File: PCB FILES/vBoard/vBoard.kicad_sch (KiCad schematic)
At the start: 209 parts, among them SW1 SW_Push, SW10 SW_Push, SW11 SW_Push, SW12 SW_Push, SW13 SW_Push, SW14 SW_Push, SW15 SW_Push, SW16 SW_Push, SW17 SW_Push, SW18 SW_Push, SW19 SW_Push, SW2 SW_Push, SW20 SW_Push, SW21 SW_Push, SW22 SW_Push, SW23 SW_Push, SW24 SW_Push, SW25 SW_Push, SW26 SW_Push, SW27 SW_Push, SW28 SW_Push, SW29 SW_Push, SW3 SW_Push, SW30 SW_Push, SW31 SW_Push, SW32 SW_Push, SW33 SW_Push, SW34 SW_Push, SW35 SW_Push, SW36 SW_Push, SW37 SW_Push, SW38 SW_Push, SW39 SW_Push, SW4 SW_Push, SW40 SW_Push, SW41 SW_Push, SW42 SW_Push, SW43 SW_Push, SW44 SW_Push, SW45 SW_Push, SW46 SW_Push, SW47 SW_Push, SW48 SW_Push, SW49 SW_Push, SW5 SW_Push, SW50 SW_Push, SW51 SW_Push, SW52 SW_Push, SW53 SW_Push, SW54 SW_Push, SW55 SW_Push, SW56 SW_Push, SW57 SW_Push, SW58 SW_Push, SW59 SW_Push, SW6 SW_Push, SW60 SW_Push, SW61 SW_Push, SW62 SW_Push, SW63 SW_Push, SW64 SW_Push, SW65 SW_Push, SW66 SW_Push, SW67 SW_Push, SW68 SW_Push, SW69 SW_Push, SW7 SW_Push, SW70 SW_Push, SW71 SW_Push, SW72 SW_Push, SW73 SW_Push, SW74 SW_Push, SW75 SW_Push, SW76 SW_Push, SW77 SW_Push, SW78 SW_Push, SW79 SW_Push, SW8 SW_Push, SW80 SW_Push, SW81 SW_Push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

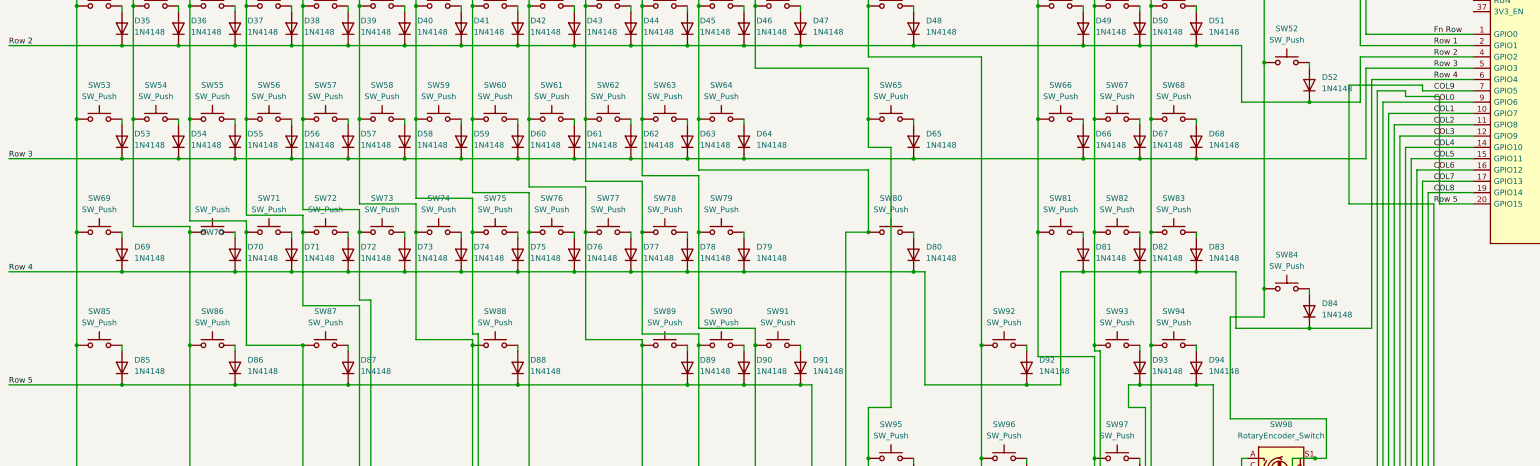
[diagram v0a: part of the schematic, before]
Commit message: DRC fixes.
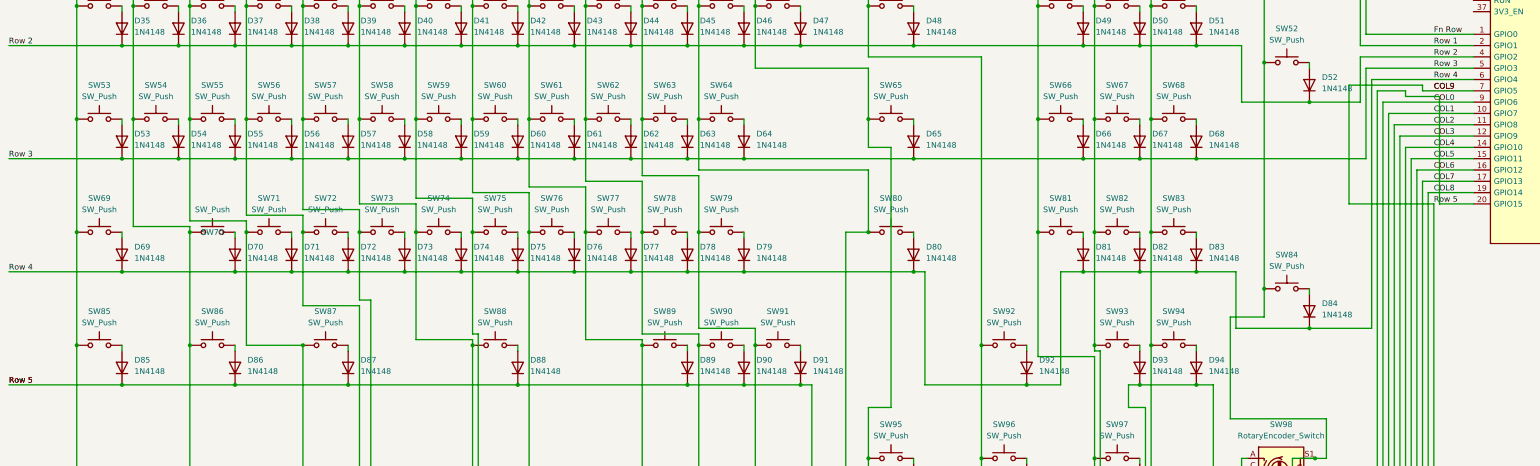
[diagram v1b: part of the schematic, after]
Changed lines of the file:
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@@
+		)
+	)
+	(label "COL9"
+		(at 332.74 99.06 0)
+		(effects
+			(font
+				(size 1.27 1.27)
+			)
+			(justify left bottom)
 		)
 	)
@@
 		)
 	)
+	(label "COL12"
+		(at 218.44 17.78 0)
+		(effects
+			(font
+				(size 1.27 1.27)
+			)
+			(justify left bottom)
+		)
+	)
+	(label "Row 5"
+		(at 12.7 165.1 0)
+		(effects
+			(font
+				(size 1.27 1.27)
+			)
+			(justify left bottom)
+		)
+	)
+	(label "COL14"
+		(at 243.84 17.78 0)
+		(effects
+			(font
+				(size 1.27 1.27)
+			)
+			(justify left bottom)
+		)
+	)
+	(label "Fn Row"
+		(at 332.74 86.36 0)
+		(effects
+			(font
+				(size 1.27 1.27)
+			)
+			(justify left bottom)
+		)
+	)
+	(label "COL5"
+		(at 332.74 114.3 0)
+		(effects
+			(font
+				(size 1.27 1.27)
+			)
+			(justify left bottom)
+		)
+	)
+	(label "COL11"
+		(at 392.43 91.44 0)
+		(effects
+			(font
+				(size 1.27 1.27)
+			)
+			(justify left bottom)
+		)
+	)
+	(label "COL10"
+		(at 193.04 17.78 0)
+		(effects
+			(font
+				(size 1.27 1.27)
+			)
+			(justify left bottom)
+		)
+	)
+	(label "COL13"
+		(at 392.43 96.52 0)
+		(effects
+			(font
+				(size 1.27 1.27)
+			)
+			(justify left bottom)
+		)
+	)
+	(label "COL12"
+		(at 392.43 93.98 0)
+		(effects
+			(font
+				(size 1.27 1.27)
+			)
+			(justify left bottom)
+		)
+	)
+	(label "Row 2"
+		(at 12.7 88.9 0)
+		(effects
+			(font
+				(size 1.27 1.27)
+			)
+			(justify left bottom)
+		)
+	)
+	(label "COL8"
+		(at 332.74 121.92 0)
+		(effects
+			(font
+				(size 1.27 1.27)
+			)
+			(justify left bottom)
+		)
+	)
+	(label "COL0"
+		(at 27.94 17.78 0)
+		(effects
+			(font
+				(size 1.27 1.27)
+			)
+			(justify left bottom)
+		)
+	)
 	(label "Row 5"
 		(at 332.74 124.46 0)
 		(effects
 			(font
-				(size 1.27 1.27)
-			)
-			(justify left bottom)
-		)
-	)
-	(label "COL12"
-		(at 218.44 17.78 0)
-		(effects
-			(font
-				(size 1.27 1.27)
-			)
-			(justify left bottom)
-		)
-	)
-	(label "COL14"
-		(at 243.84 17.78 0)
-		(effects
-			(font
-				(size 1.27 1.27)
-			)
-			(justify left bottom)
-		)
-	)
-	(label "Fn Row"
-		(at 332.74 86.36 0)
-		(effects
-			(font
-				(size 1.27 1.27)
-			)
-			(justify left bottom)
-		)
-	)
-	(label "COL5"
-		(at 332.74 114.3 0)
-		(effects
-			(font
-				(size 1.27 1.27)
-			)
-			(justify left bottom)
-		)
-	)
-	(label "COL11"
-		(at 392.43 91.44 0)
-		(effects
-			(font
-				(size 1.27 1.27)
-			)
-			(justify left bottom)
-		)
-	)
-	(label "COL10"
-		(at 193.04 17.78 0)
-		(effects
-			(font
-				(size 1.27 1.27)
-			)
-			(justify left bottom)
-		)
-	)
-	(label "COL13"
-		(at 392.43 96.52 0)
-		(effects
-			(font
-				(size 1.27 1.27)
-			)
-			(justify left bottom)
-		)
-	)
-	(label "COL12"
-		(at 392.43 93.98 0)
-		(effects
-			(font
-				(size 1.27 1.27)
-			)
-			(justify left bottom)
-		)
-	)
-	(label "Row 2"
-		(at 12.7 88.9 0)
-		(effects
-			(font
-				(size 1.27 1.27)
-			)
-			(justify left bottom)
-		)
-	)
-	(label "COL8"
-		(at 332.74 121.92 0)
-		(effects
-			(font
-				(size 1.27 1.27)
-			)
-			(justify left bottom)
-		)
-	)
-	(label "COL0"
-		(at 27.94 17.78 0)
-		(effects
-			(font
